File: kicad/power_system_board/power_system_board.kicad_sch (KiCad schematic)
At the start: 20 parts, among them J1 USB_B_Micro, J2 Conn_01x04_Pin, J3 Conn_01x02_Pin, J4 Conn_01x02_Pin, J5 Conn_01x02_Pin, J6 Conn_01x02_Pin, Q1 2N7002H, Q2 2N7002H, U1 MCP73831-2-OT, U3 AP9101CK6

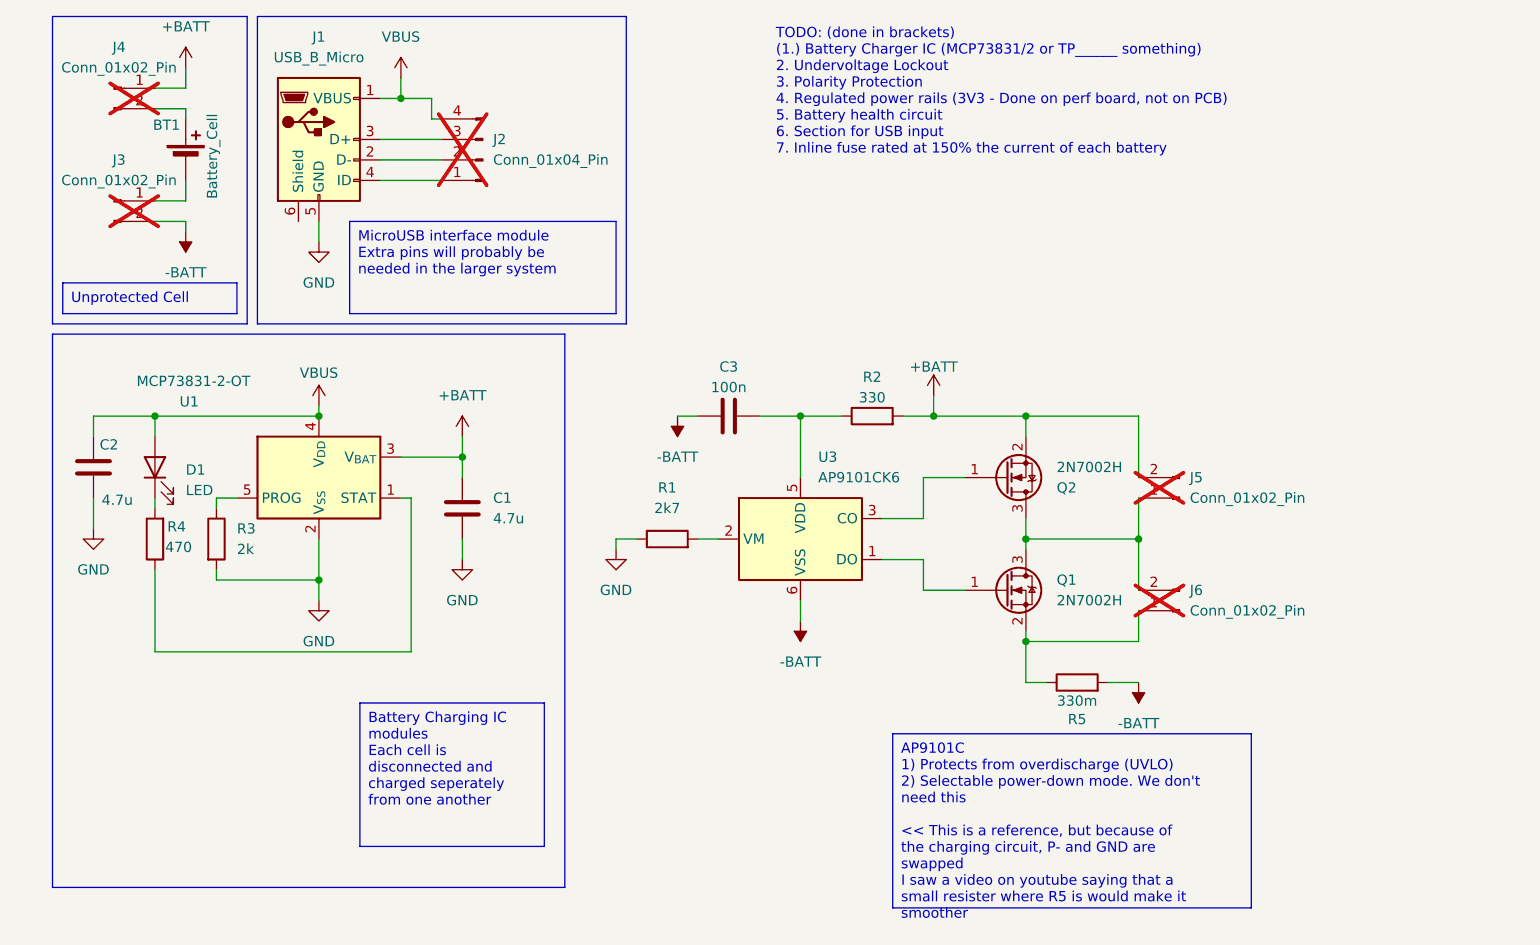
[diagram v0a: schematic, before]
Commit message: Checkpoint
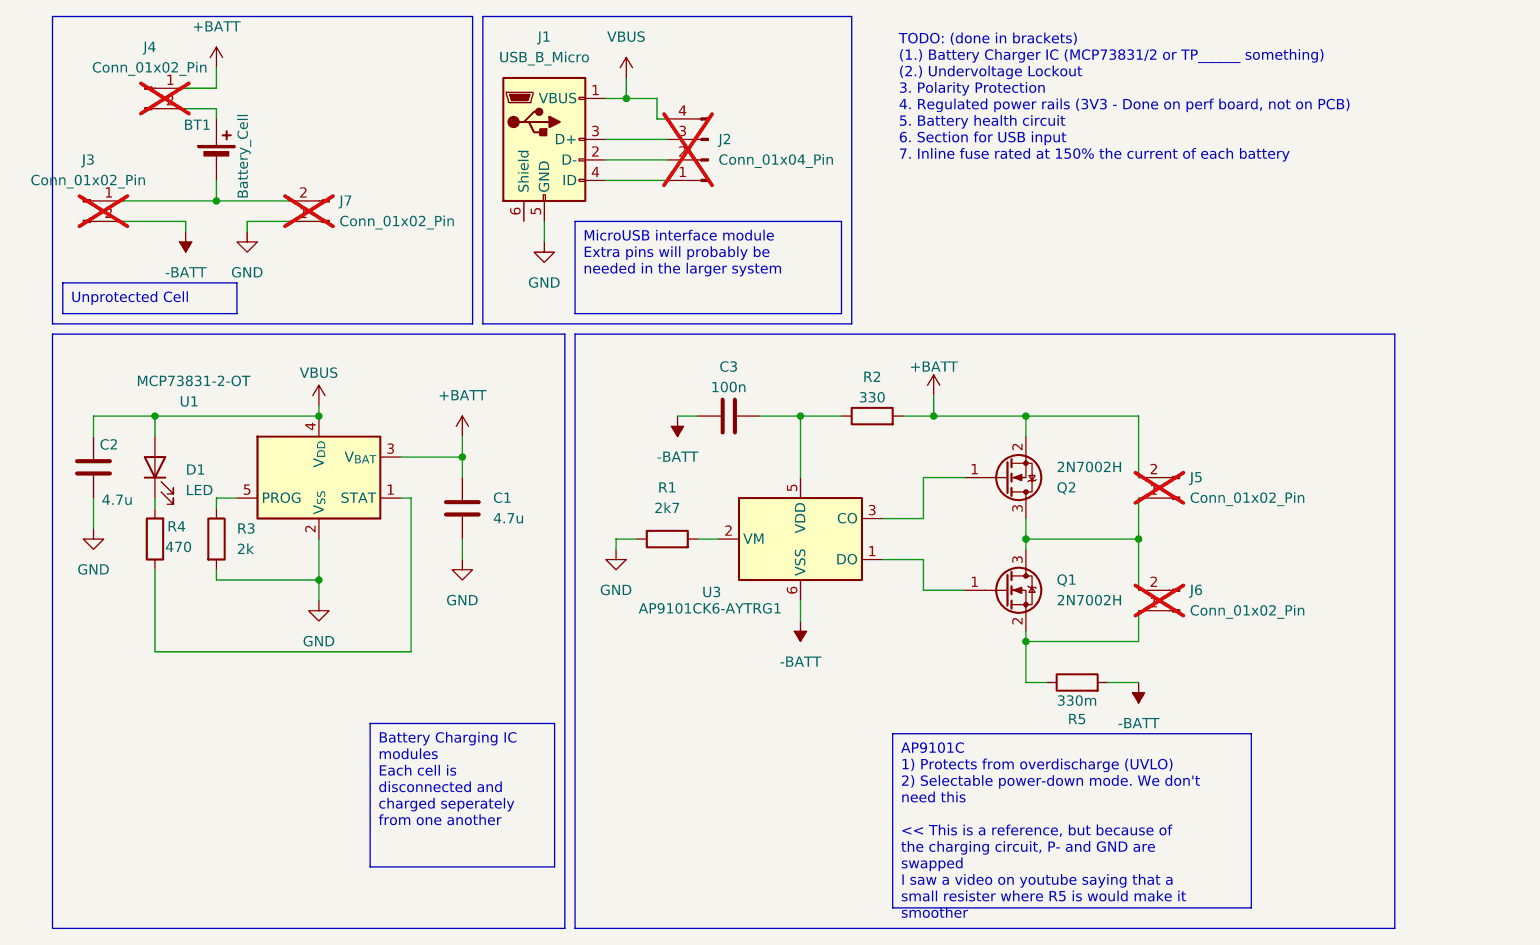
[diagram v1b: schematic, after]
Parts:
- added J7: Conn_01x02_Pin, Connector_PinHeader_2.54mm:PinHeader_1x02_P2.54mm_Vertical, symbol Connector:Conn_01x02_Pin
- U3: value AP9101CK6 -> AP9101CK6-AYTRG1
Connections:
- net GND: now also J7.1 (Pin_1)
- net at BT1.2 (-), J3.1 (Pin_1): now also J7.2 (Pin_2)
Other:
- note added: "TODO: (done in brackets) (1.) Battery Charger IC (MCP73831/2 or TP______ something) (2.) Undervoltage Lockout 3. Polarity Protection 4. Regulated power rails (3V3 - Done on perf board, not on PCB) 5. Battery health circuit 6. Section for USB input 7. Inline fuse rated at 150% the current of each battery"
- note removed: "TODO: (done in brackets) (1.) Battery Charger IC (MCP73831/2 or TP______ something) 2. Undervoltage Lockout 3. Polarity Protection 4. Regulated power rails (3V3 - Done on perf board, not on PCB) 5. Battery health circuit 6. Section for USB input 7. Inline fuse rated at 150% the current of each battery"
- moved on the sheet: BT1, J1, J2, J3, J4
